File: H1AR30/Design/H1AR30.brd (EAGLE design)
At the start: 34.6 x 30 mm, 21 parts, among them P1 HEXABIT_17.32_NO_P3, U1 STM32F091CBU6, X1 XTALL_CSTCE8M00G52

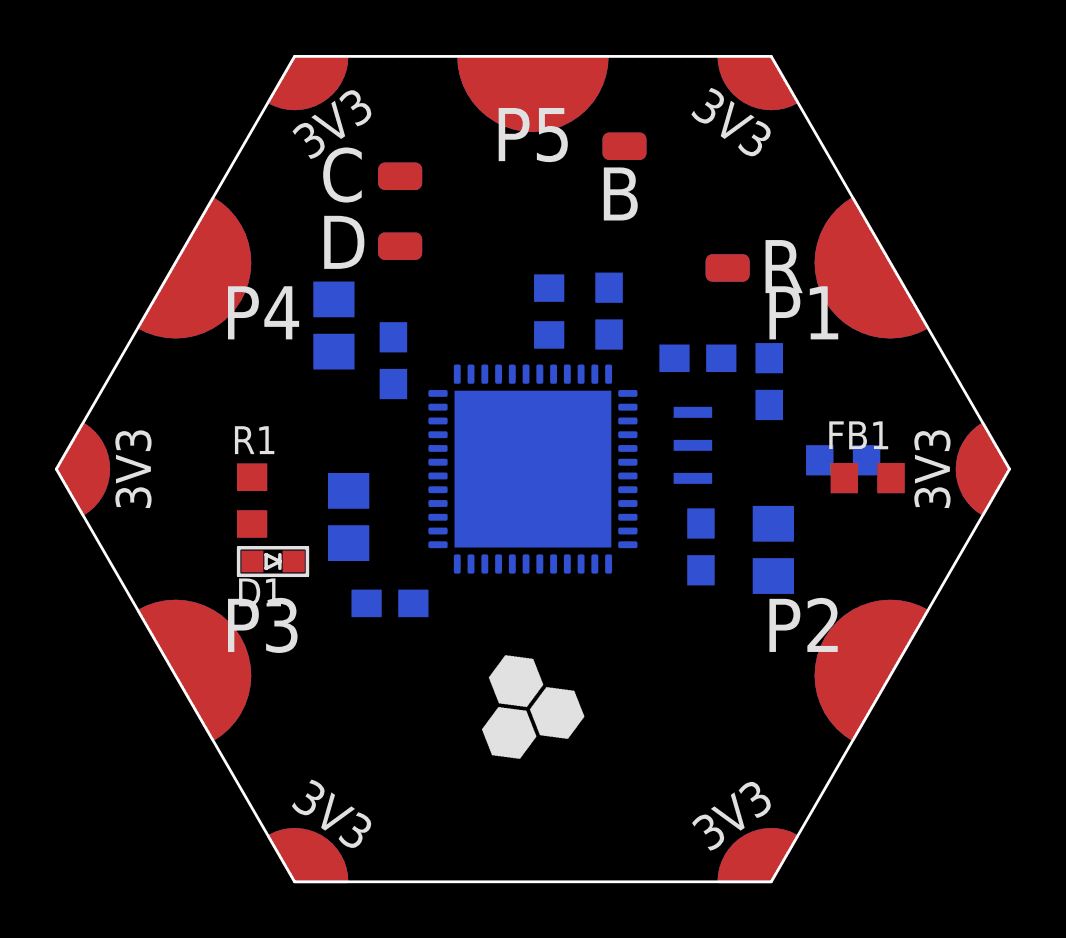
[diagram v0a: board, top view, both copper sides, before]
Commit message: in this commit: - schematic is done - PCB is done - all output files were generated
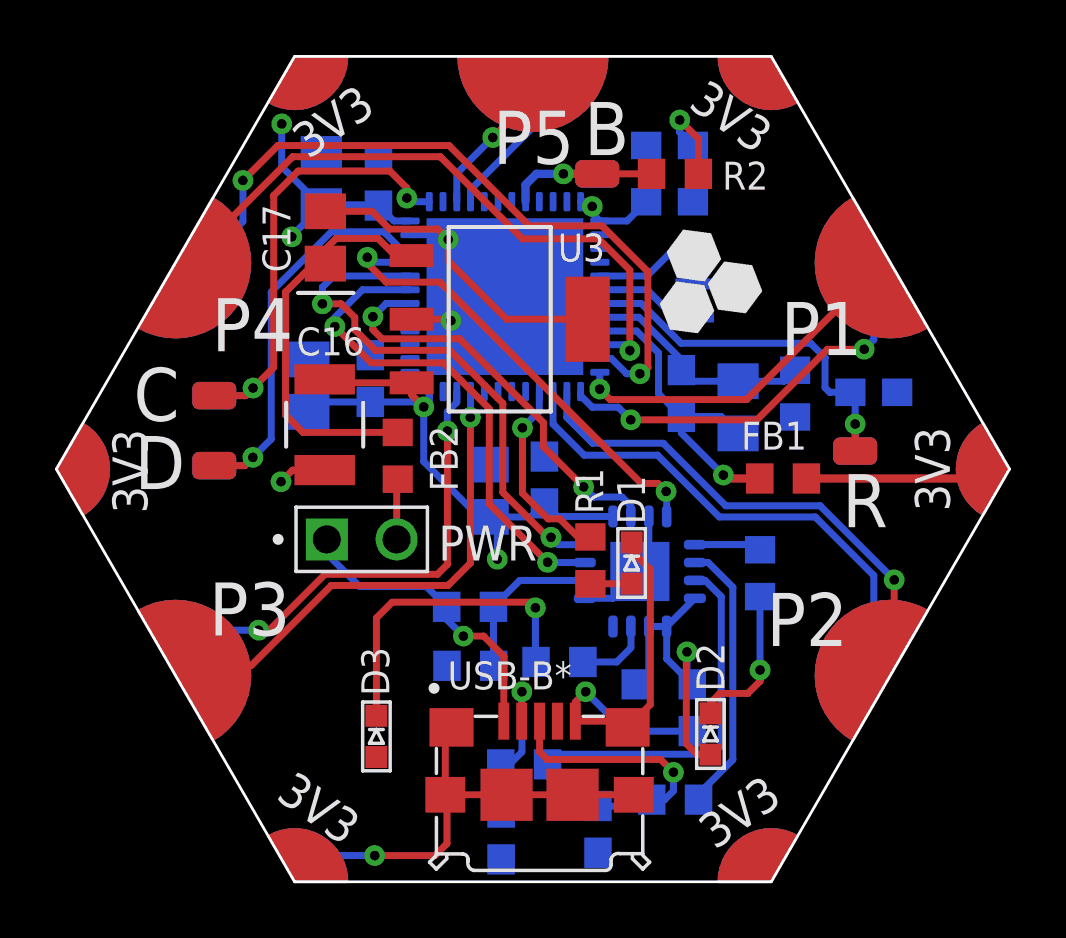
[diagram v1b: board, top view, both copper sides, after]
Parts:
- added C10: 4.7uF, Hexabitz:C-0805-POL
- added C11, C12, C15: 100nF, Hexabitz:C-0603
- added C13, C14: 47pF, Hexabitz:C-0603
- added C16: 100uF, Hexabitz:C-3225
- added C17: 1uF, Hexabitz:C-0805-POL
- added D2: RED, Hexabitz:VLMS1300-GS08
- added D3: GREEN, Hexabitz:VLMS1300-GS08
- added FB2: (no value), Hexabitz:FB-TDK_MMZ1608Y300B
- added PWR: 3-644456-2, Hexabitz:TE_3-644456-2
- added R4, R5: 27.0Ω, Hexabitz:R-0603
- added R6: 39.0Ω, Hexabitz:R-0603
- added R7: 270.0Ω, Hexabitz:R-0603
- added R8: 4.7kΩ, Hexabitz:R-0603
- added R9: 10kΩ, Hexabitz:R-0603
- added U2: FT230XQ-R, Hexabitz:QFN16
- added U3: LM3940IMP-3.3, Hexabitz:SOT230P696X180-4N
- added USB-B*: 1981568-1, Hexabitz:TE_1981568-1
- C1: value 10nF -> 100nF
- C3: value 100nF -> 4.7uF; device Hexabitz:C-0603 -> Hexabitz:C-0805-POL
- C5: value 100nF -> 10nF
- C7: value 4.7uF -> 100nF; device Hexabitz:C-0805-POL -> Hexabitz:C-0603
- D1: value VLMS1300-GS08 -> RED
- R2: value 0.0R -> 10.0K
- R3: value 10.0K -> 0.0R
- moved C6 15.3 mm to (29.0, 45.0), turned to 90 degrees
- moved C8 14.5 mm to (28.7, 37.9)
- moved C7 13.8 mm to (39.6, 46.4), turned to 180 degrees
- moved D1 13.0 mm to (38.2, 31.2), turned to 180 degrees
- moved R1 12.5 mm to (36.7, 31.3)
- moved R2 12.1 mm to (39.8, 45.4), flipped to the top, turned to 180 degrees
- moved C3 11.5 mm to (26.9, 45.1)
- moved C5 10.5 mm to (40.0, 37.4)
- moved D 10.5 mm to (23.0, 34.7)
- moved C 10.5 mm to (23.0, 37.3)
- moved R3 9.42 mm to (44.1, 37.4), turned to 90 degrees
- moved C1 8.43 mm to (47.0, 37.4), turned to 180 degrees
- moved R 8.11 mm to (46.3, 35.3)
- moved U1 6.35 mm to (33.6, 40.9)
- moved X1 5.87 mm to (40.5, 41.3)
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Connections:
- new net N$1: R1.2, U1.P$16
- new net N$10: FB2.2, PWR.2
- new net N$11: C17.1, FB2.1, U3.1
- new net N$12: R5.2, U2.6
- new net N$13: R4.2, U2.7
- new net N$14: R7.1, U2.5
- new net N$15: R6.1, U2.11
- new net N$16: D2.C, R7.2
- new net N$17: D3.C, R6.2
- new net N$18: PWR.1, R8.2, USB-B*.1
- new net N$2: C14.1, R4.1, USB-B*.2
- new net UART1_CTS: U1.P$32, U2.16
- new net UART1_RTS: U1.P$33, U2.4
- new net VBUS_SENSE: R8.1, R9.2, U2.14
- net B1: now also R2.2; no longer R3.2
- net GND: now also C1.2, C10.2, C11.2, C12.2, C13.2, C14.2, C15.2, C16.1, C17.2, R9.1, U1.P$19, U1.P$27, U1.P$3, U1.P$38, U2.13, U2.17, U2.3, U3.2, U3.4, USB-B*.10, USB-B*.11, USB-B*.5, USB-B*.6, USB-B*.7, USB-B*.8, USB-B*.9; no longer C5.2
- net N$3: now also C13.1, R5.1, USB-B*.3; no longer R1.2, U1.P$32
- net R1: now also C1.1; no longer C8.1
- net UART1_RX: now also U2.15
- net UART1_TX: now also U2.2
- net UART2_RX: now also P1.PAD_PD1
- net UART2_TX: now also P1.PAD_PU1
- net UART3_RX: now also P1.PAD_PD4
- net UART3_TX: now also P1.PAD_PU4
- net UART4_RX: now also P1.PAD_PD5
- net UART4_TX: now also P1.PAD_PU5
- net UART5_RX: now also P1.PAD_PD6
- net UART5_TX: now also P1.PAD_PU6
- net UART6_RX: now also P1.PAD_PD2
- net UART6_TX: now also P1.PAD_PU2
- net VDD: now also C10.1, C11.1, C12.1, C15.1, C16.2, C8.1, D2.A, D3.A, U2.1, U2.10, U2.8, U2.9, U3.3; no longer C5.1
- net VDDA: now also C5.1; no longer C1.1
- net VSSA: now also C5.2, R3.2; no longer C1.2, R2.2
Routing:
- net GND: track 0.00 -> 58.8 mm, vias 0 -> 6
- net VDD: track 0.00 -> 54.1 mm, vias 0 -> 6
- net UART4_RX: track 0.00 -> 26.8 mm, vias 0 -> 2
- net UART4_TX: track 0.00 -> 23.8 mm, vias 0 -> 1
- net UART1_CTS: track 0.00 -> 19.3 mm, vias 0 -> 2
- net UART6_TX: track 0.00 -> 18.7 mm, vias 0 -> 1
- net UART6_RX: track 0.00 -> 18.4 mm
- net UART1_RX: track 0.00 -> 18.2 mm, vias 0 -> 2
- net UART3_TX: track 0.00 -> 17.9 mm, vias 0 -> 1
- net UART3_RX: track 0.00 -> 17.2 mm, vias 0 -> 2
- net N$9: track 0.00 -> 17.1 mm, vias 0 -> 2
- net UART1_RTS: track 0.00 -> 17.1 mm, vias 0 -> 2
- net N$7: track 0.00 -> 15.5 mm, vias 0 -> 1
- net UART1_TX: track 0.00 -> 14.9 mm, vias 0 -> 2
- net UART2_RX: track 0.00 -> 14.8 mm, vias 0 -> 2
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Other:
- board text added: "H1AR20"
- board text removed: "H1AR30"
